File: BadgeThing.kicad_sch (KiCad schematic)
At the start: 65 parts, among them J1 USB_C_Receptacle_USB2.0, J2 Connector_Generic_Conn_01x02, J3 Ext 5V, J4 SWD Header, J6 Conn_01x07, J7 Conn_01x07, J8 Conn_01x08, SW1 BOOTSEL, SW2 ESP RESET, SW3 Left, SW4 Down, SW5 Select, SW6 Up, SW7 Right, U2 W25Q32JVSS, U3 RP2040, U4 NCP1117-3.3_SOT223, U5 ESP-12F, Y1 12.000MHz

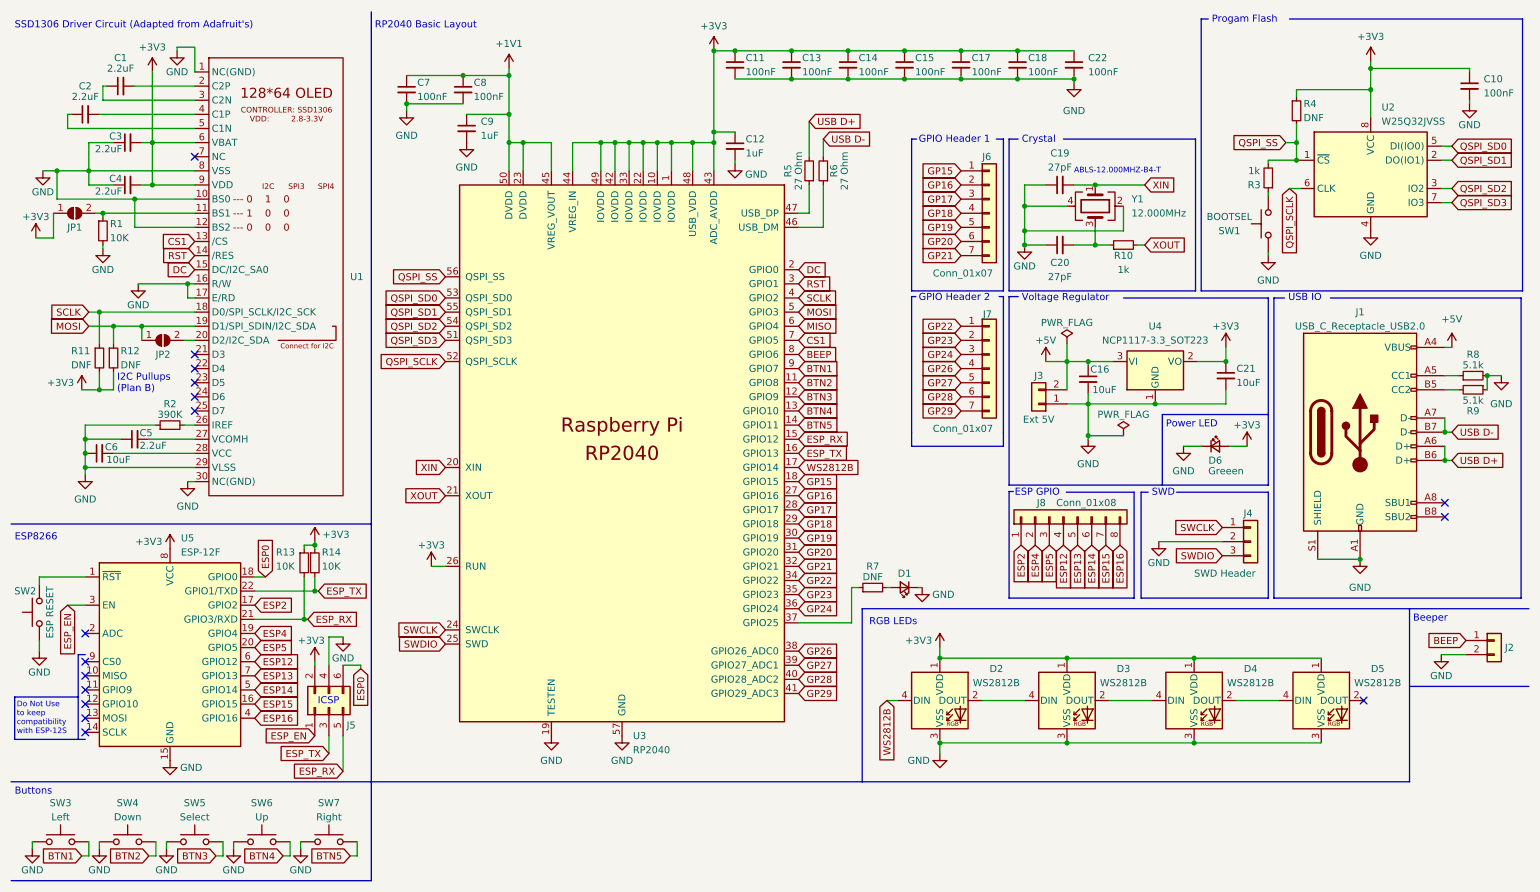
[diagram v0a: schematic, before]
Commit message: more routing + layout
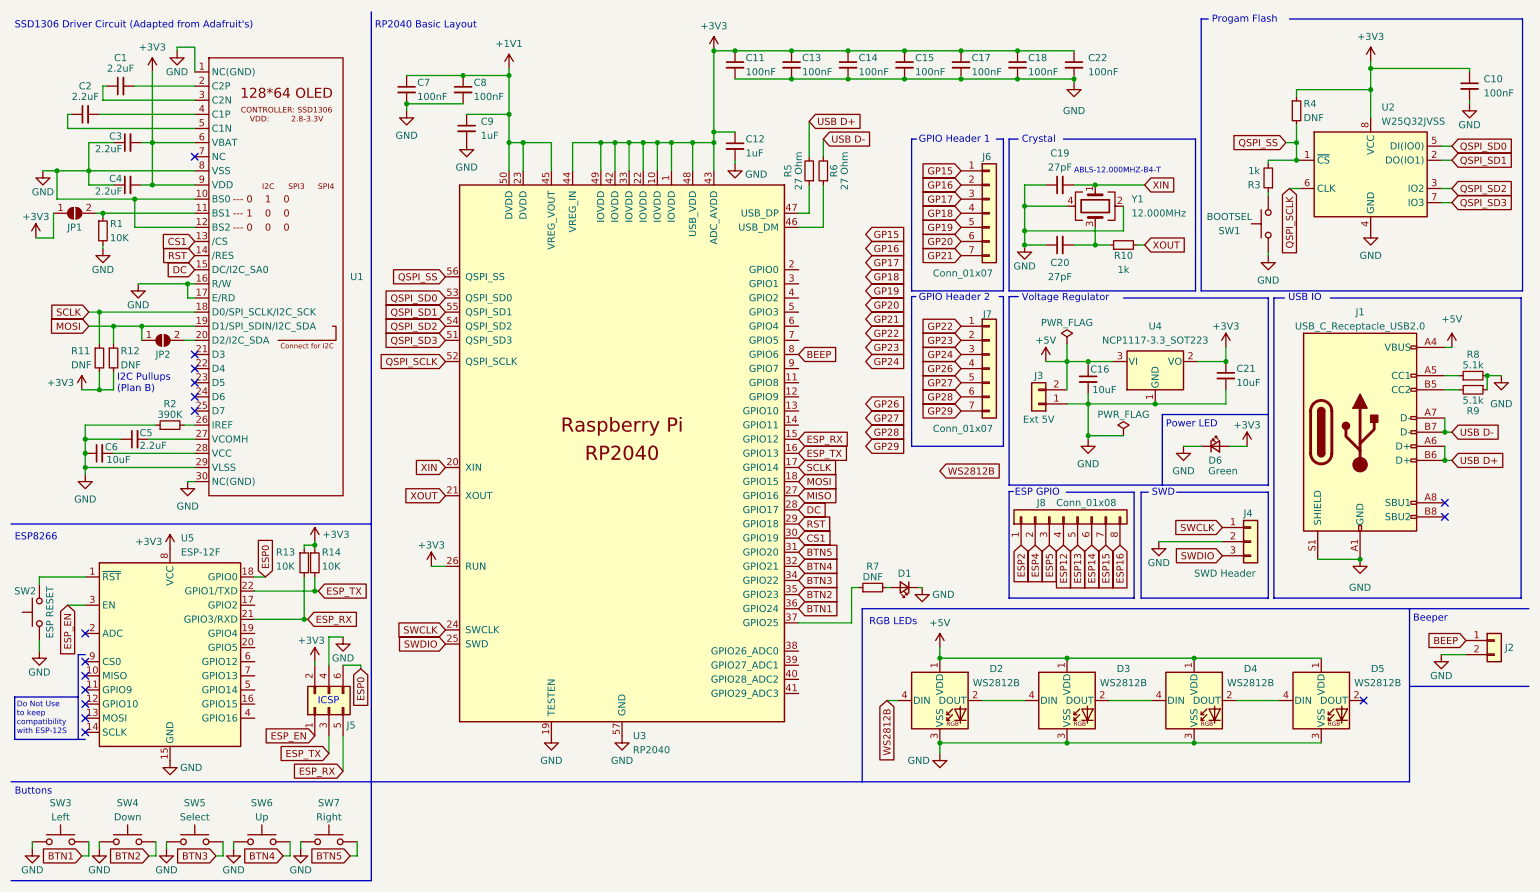
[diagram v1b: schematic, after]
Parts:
- D6: value Greeen -> Green
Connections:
- net +3V3: no longer D2.1 (VDD), D3.1 (VDD), D4.1 (VDD), D5.1 (VDD)
- net +5V: now also D2.1 (VDD), D3.1 (VDD), D4.1 (VDD), D5.1 (VDD)
- net BTN1: now also U3.36 (GPIO24); no longer U3.9 (GPIO7)
- net BTN2: now also U3.35 (GPIO23); no longer U3.11 (GPIO8)
- net BTN3: now also U3.34 (GPIO22); no longer U3.12 (GPIO9)
- net BTN4: now also U3.32 (GPIO21); no longer U3.13 (GPIO10)
- net BTN5: now also U3.31 (GPIO20); no longer U3.14 (GPIO11)
- net CS1: now also U3.30 (GPIO19); no longer U3.7 (GPIO5)
- net DC: now also U3.28 (GPIO17); no longer U3.2 (GPIO0)
- net ESP12: no longer U5.6 (GPIO12)
- net ESP13: no longer U5.7 (GPIO13)
- net ESP14: no longer U5.5 (GPIO14)
- net ESP15: no longer U5.16 (GPIO15)
- net ESP16: no longer U5.4 (GPIO16)
- net ESP2: no longer U5.17 (GPIO2)
- net ESP4: no longer U5.19 (GPIO4)
- net ESP5: no longer U5.20 (GPIO5)
- net GP15: no longer U3.18 (GPIO15)
- net GP16: no longer U3.27 (GPIO16)
- net GP17: no longer U3.28 (GPIO17)
- net GP18: no longer U3.29 (GPIO18)
- net GP19: no longer U3.30 (GPIO19)
- net GP20: no longer U3.31 (GPIO20)
- net GP21: no longer U3.32 (GPIO21)
- net GP22: no longer U3.34 (GPIO22)
- net GP23: no longer U3.35 (GPIO23)
- net GP24: no longer U3.36 (GPIO24)
- net GP26: no longer U3.38 (GPIO26_ADC0)
- net GP27: no longer U3.39 (GPIO27_ADC1)
- net GP28: no longer U3.40 (GPIO28_ADC2)
- net GP29: no longer U3.41 (GPIO29_ADC3)
- net MISO: now also U3.27 (GPIO16); no longer U3.6 (GPIO4)
- net MOSI: now also U3.18 (GPIO15); no longer U3.5 (GPIO3)
- net RST: now also U3.29 (GPIO18); no longer U3.3 (GPIO1)
- net SCLK: now also U3.17 (GPIO14); no longer U3.4 (GPIO2)
- net WS2812B: no longer U3.17 (GPIO14)
